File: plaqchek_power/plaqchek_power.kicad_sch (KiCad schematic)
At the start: 31 parts, among them J1 Conn_01x05, J2 Conn_01x04, J3 Barrel_Jack_Switch, J4 Conn_01x03

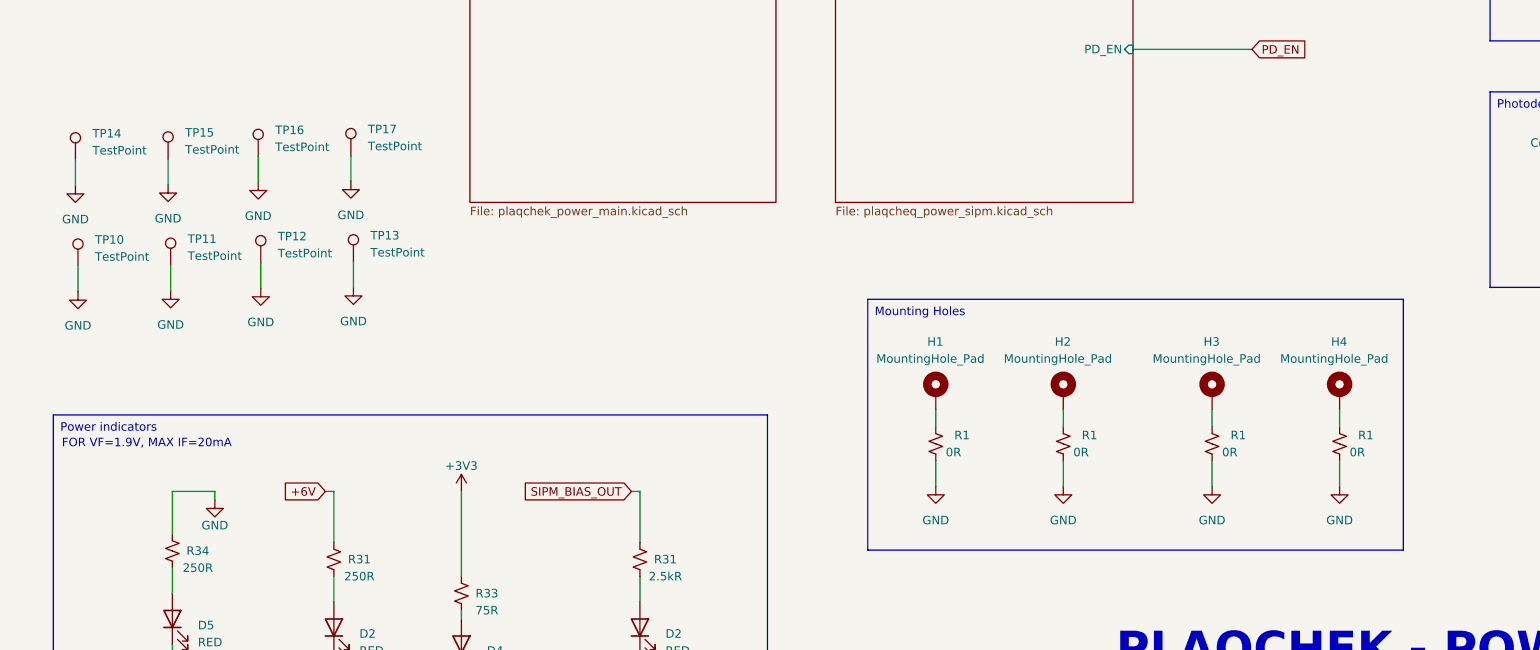
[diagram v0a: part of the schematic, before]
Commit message: finish all pcbs, generate gerber files
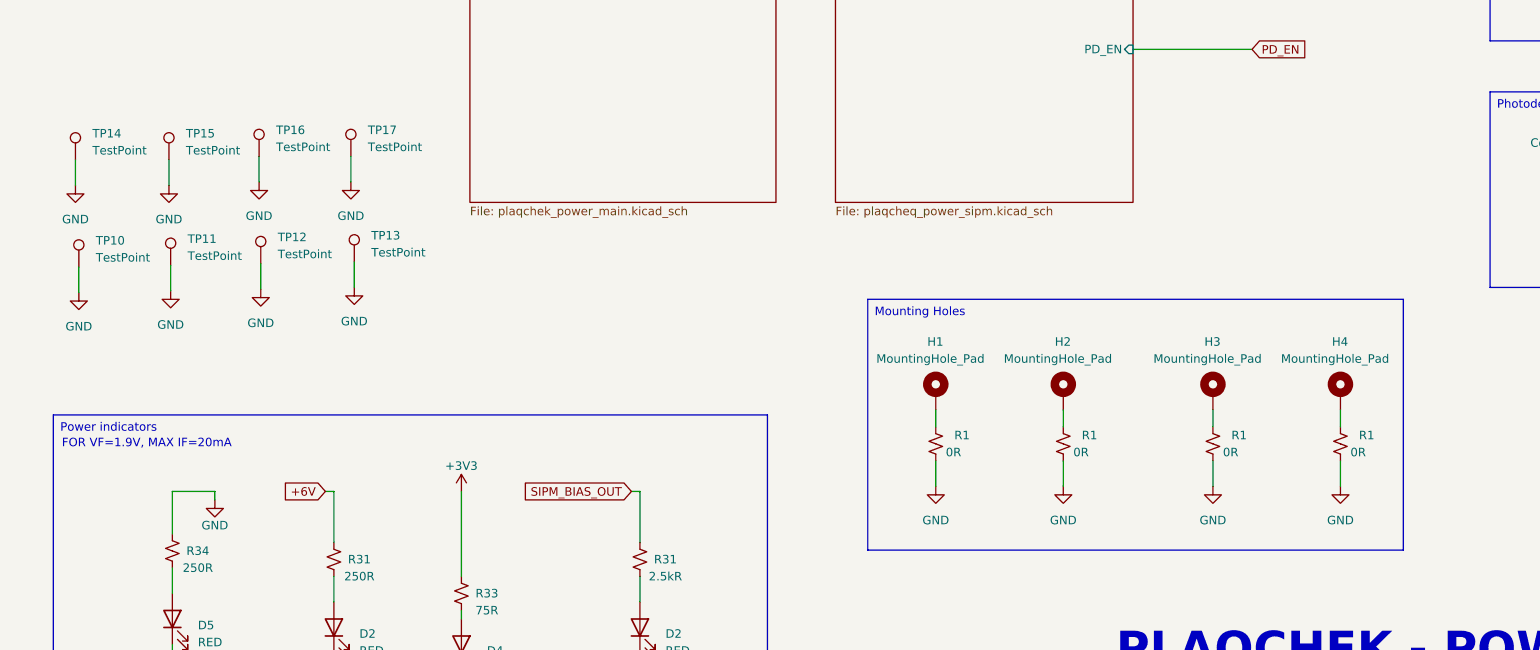
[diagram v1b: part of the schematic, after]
